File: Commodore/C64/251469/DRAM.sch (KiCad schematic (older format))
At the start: 24 parts, among them U10 4164, U11 4164, U12 4164, U21 4164, U22 4164, U23 4164, U24 4164, U9 4164

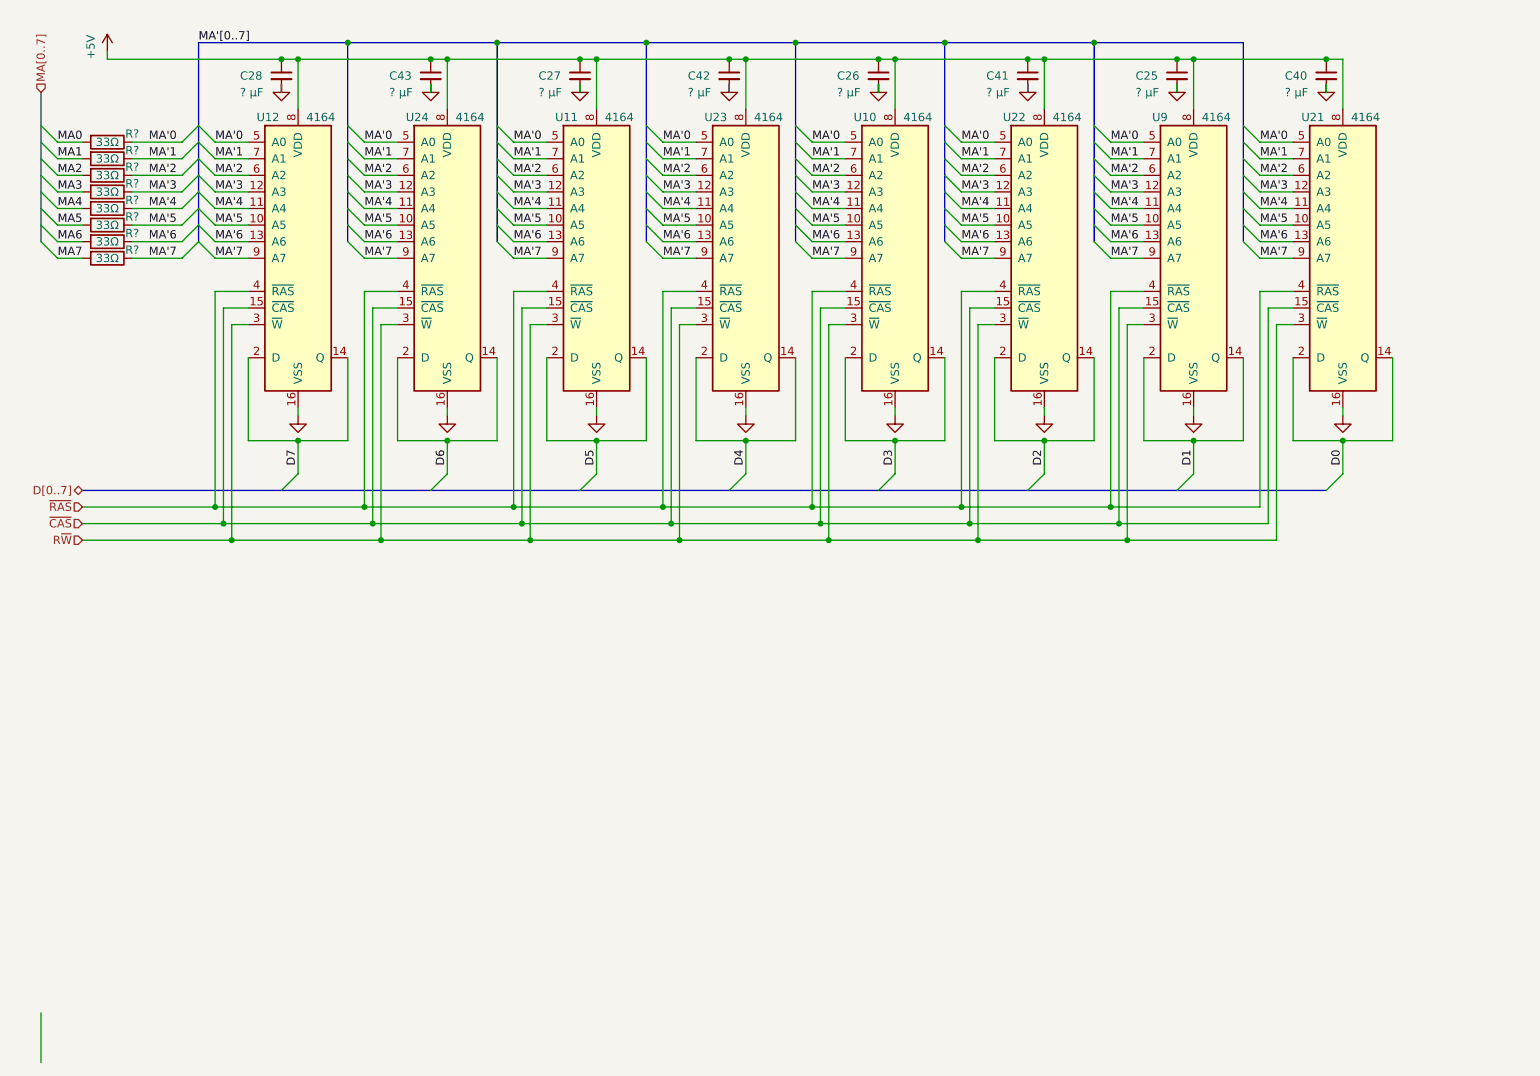
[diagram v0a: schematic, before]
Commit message: WIP
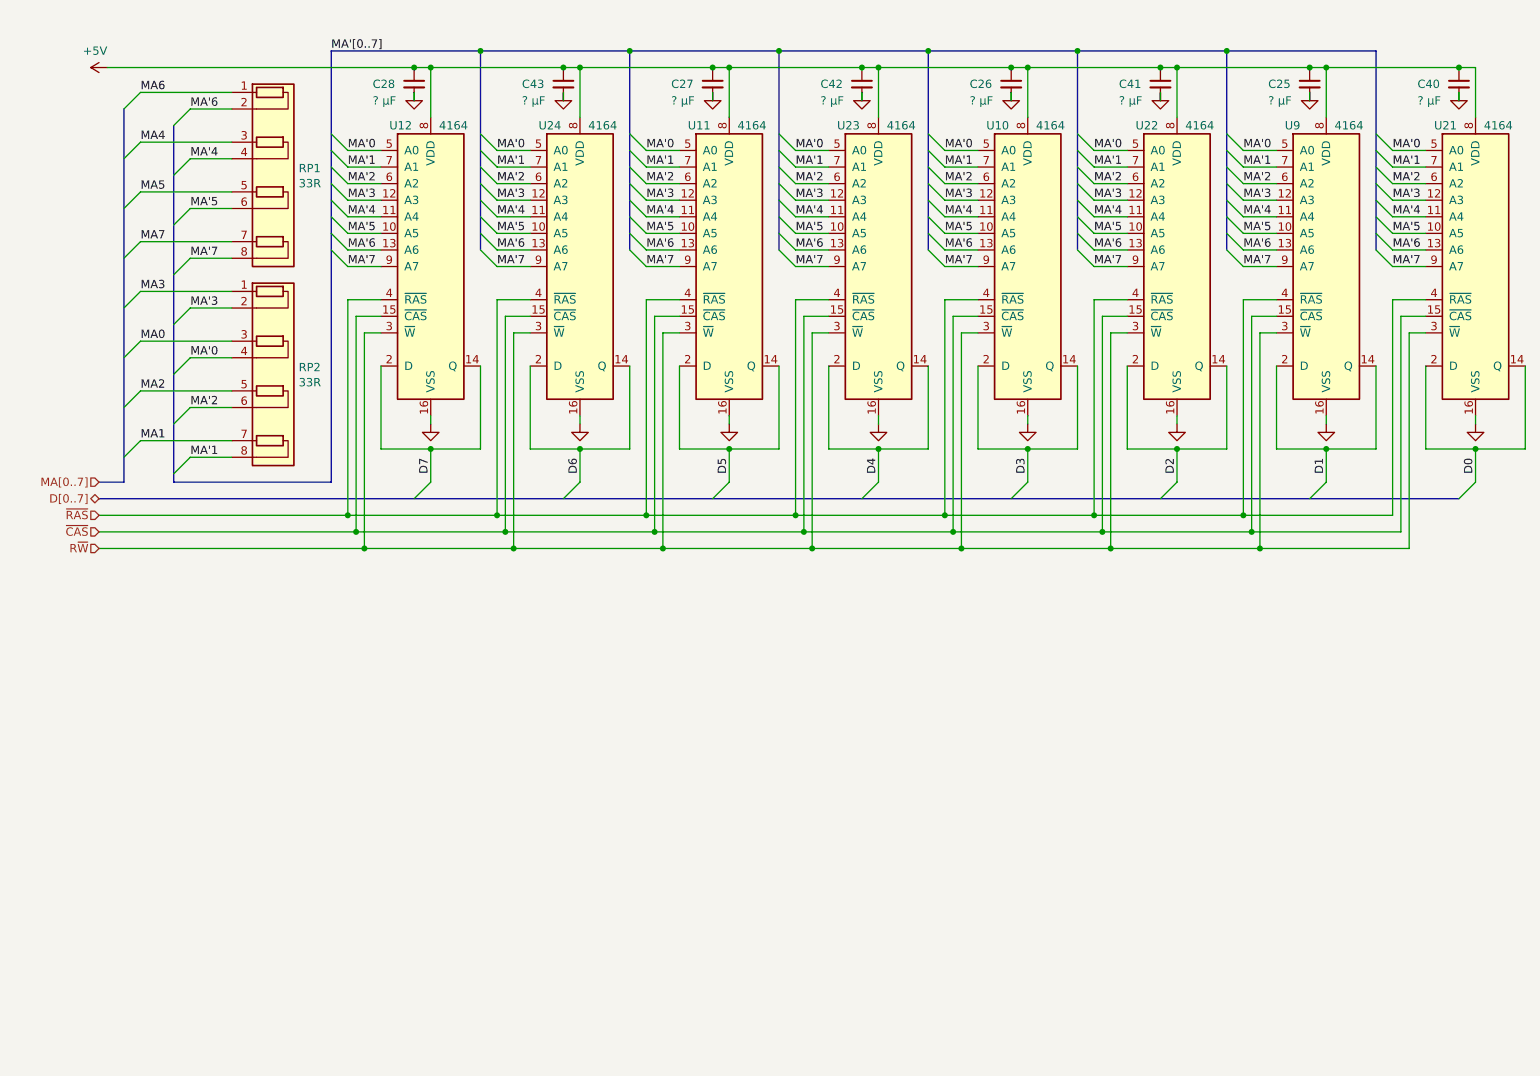
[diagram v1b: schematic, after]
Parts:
- removed R? (x8): 33Ω, symbol Device:R
- added RP1, RP2: 33R, Resistor_THT:R_Array_SIP8, symbol Device:R_Pack04_SIP
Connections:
- net MA'0: now also RP2.4 (R2.2)
- net MA'1: now also RP2.8 (R4.2)
- net MA'2: now also RP2.6 (R3.2)
- net MA'3: now also RP2.2 (R1.2)
- net MA'4: now also RP1.4 (R2.2)
- net MA'5: now also RP1.6 (R3.2)
- net MA'6: now also RP1.2 (R1.2)
- net MA'7: now also RP1.8 (R4.2)
- net MA0: now also RP2.3 (R2.1)
- net MA1: now also RP2.7 (R4.1)
- net MA2: now also RP2.5 (R3.1)
- net MA3: now also RP2.1 (R1.1)
- net MA4: now also RP1.3 (R2.1)
- net MA5: now also RP1.5 (R3.1)
- net MA6: now also RP1.1 (R1.1)
- net MA7: now also RP1.7 (R4.1)
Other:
- moved on the sheet: C25, C26, C27, C28, C40, C41, C42, C43, U10, U11, U12, U21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
